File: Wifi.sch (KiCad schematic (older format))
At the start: 15 parts

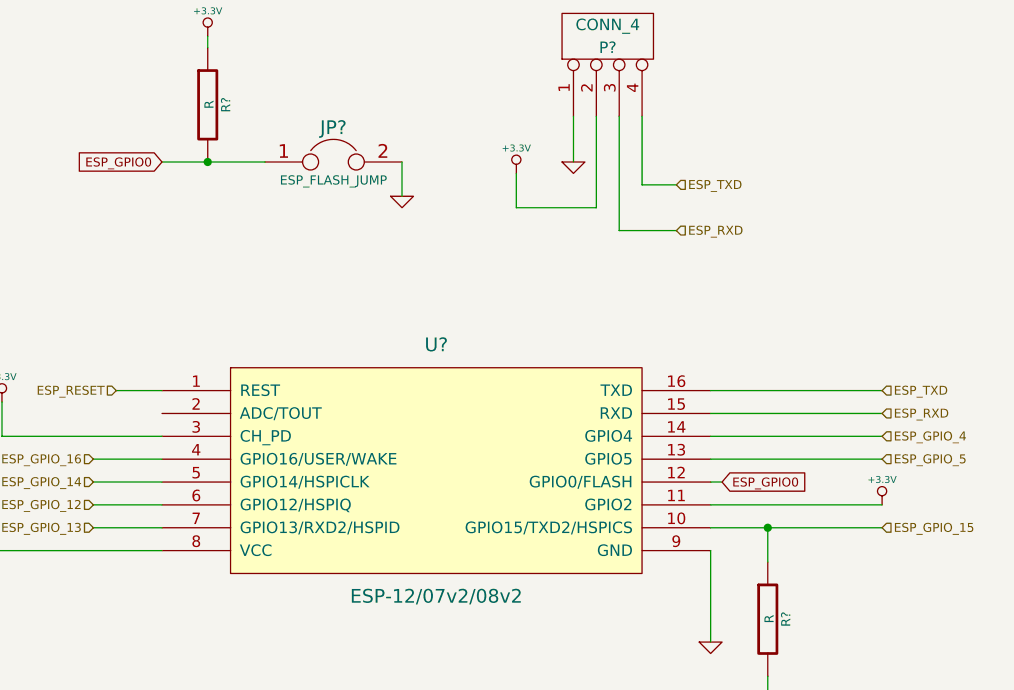
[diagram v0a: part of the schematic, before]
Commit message: Think sch finished
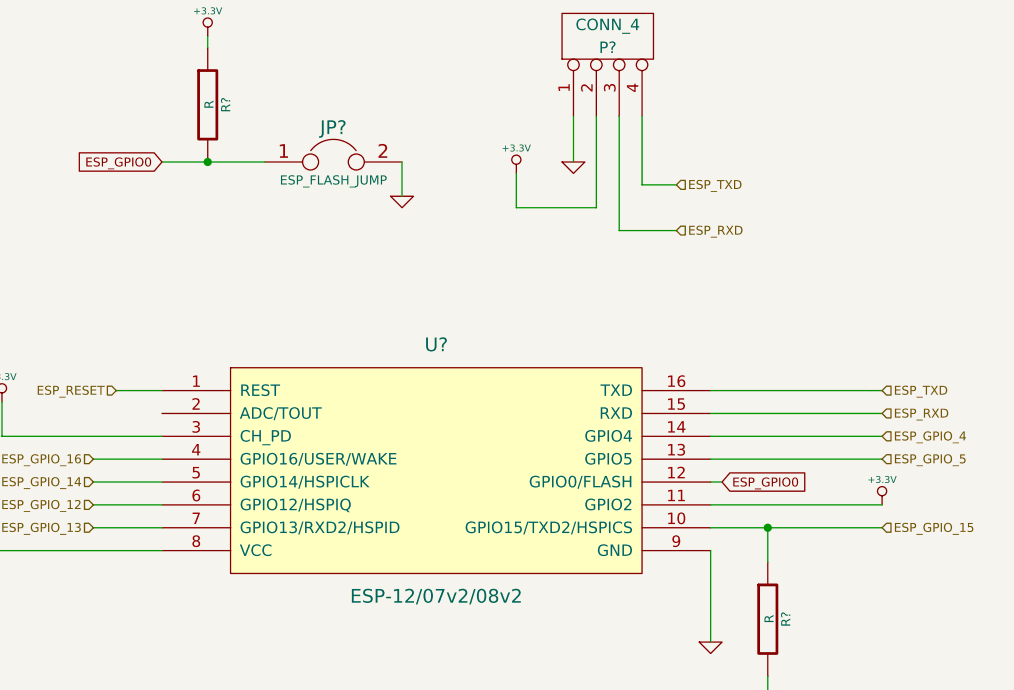
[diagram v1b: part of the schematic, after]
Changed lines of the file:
@@
 $EndComp
 $Comp
-L GND #PWR?
+L GND #PWR054
 U 1 1 55667722
 P 6650 2900
-F 0 "#PWR?" H 6650 2900 30  0001 C CNN
+F 0 "#PWR054" H 6650 2900 30  0001 C CNN
 F 1 "GND" H 6650 2830 30  0001 C CNN
 F 2 "" H 6650 2900 60  0000 C CNN
@@
 $EndComp
 $Comp
-L +3.3V #PWR?
+L +3.3V #PWR055
 U 1 1 55667729
 P 6400 2950
-F 0 "#PWR?" H 6400 2910 30  0001 C CNN
+F 0 "#PWR055" H 6400 2910 30  0001 C CNN
 F 1 "+3.3V" H 6400 3060 30  0000 C CNN
 F 2 "" H 6400 2950 60  0000 C CNN
@@
 $EndComp
 $Comp
-L +3.3V #PWR?
+L +3.3V #PWR056
 U 1 1 55667746
 P 5050 2350
-F 0 "#PWR?" H 5050 2310 30  0001 C CNN
+F 0 "#PWR056" H 5050 2310 30  0001 C CNN
 F 1 "+3.3V" H 5050 2460 30  0000 C CNN
 F 2 "" H 5050 2350 60  0000 C CNN
@@
 $EndComp
 $Comp
-L GND #PWR?
+L GND #PWR057
 U 1 1 5566774C
 P 5900 3050
-F 0 "#PWR?" H 5900 3050 30  0001 C CNN
+F 0 "#PWR057" H 5900 3050 30  0001 C CNN
 F 1 "GND" H 5900 2980 30  0001 C CNN
 F 2 "" H 5900 3050 60  0000 C CNN
@@
 ESP8266 Wifi Module
 $Comp
-L +3.3V #PWR?
+L +3.3V #PWR058
 U 1 1 5566775A
 P 8000 4400
-F 0 "#PWR?" H 8000 4360 30  0001 C CNN
+F 0 "#PWR058" H 8000 4360 30  0001 C CNN
 F 1 "+3.3V" H 8000 4510 30  0000 C CNN
 F 2 "" H 8000 4400 60  0000 C CNN
@@
 $EndComp
 $Comp
-L +3.3V #PWR?
+L +3.3V #PWR059
 U 1 1 55667760
 P 4150 3950
-F 0 "#PWR?" H 4150 3910 30  0001 C CNN
+F 0 "#PWR059" H 4150 3910 30  0001 C CNN
 F 1 "+3.3V" H 4150 4060 30  0000 C CNN
 F 2 "" H 4150 3950 60  0000 C CNN
@@
 $EndComp
 $Comp
-L GND #PWR?
+L GND #PWR060
 U 1 1 5566776E
 P 7500 5350
-F 0 "#PWR?" H 7500 5350 30  0001 C CNN
+F 0 "#PWR060" H 7500 5350 30  0001 C CNN
 F 1 "GND" H 7500 5280 30  0001 C CNN
 F 2 "" H 7500 5350 60  0000 C CNN
@@
 $EndComp
 $Comp
-L +3.3V #PWR?
+L +3.3V #PWR061
 U 1 1 5566915C
 P 2750 4500
-F 0 "#PWR?" H 2750 4460 30  0001 C CNN
+F 0 "#PWR061" H 2750 4460 30  0001 C CNN
 F 1 "+3.3V" H 2750 4610 30  0000 C CNN
 F 2 "" H 2750 4500 60  0000 C CNN
@@
 $EndComp
 $Comp
-L GND #PWR?
+L GND #PWR062
 U 1 1 556691BF
 P 7250 5000
-F 0 "#PWR?" H 7250 5000 30  0001 C CNN
+F 0 "#PWR062" H 7250 5000 30  0001 C CNN
 F 1 "GND" H 7250 4930 30  0001 C CNN
 F 2 "" H 7250 5000 60  0000 C CNN
@@
 $EndComp
 $Comp
-L GND #PWR?
+L GND #PWR063
 U 1 1 5566925F
 P 3200 5000
-F 0 "#PWR?" H 3200 5000 30  0001 C CNN
+F 0 "#PWR063" H 3200 5000 30  0001 C CNN
 F 1 "GND" H 3200 4930 30  0001 C CNN
 F 2 "" H 3200 5000 60  0000 C CNN
@@
 	5050 2350 5050 2400
 Wire Wire Line
-	4850 2900 5300 2900
+	4850 2900 5050 2900
+Wire Wire Line
+	5050 2900 5300 2900
 Wire Wire Line
 	5900 2900 5900 3050
@@
 	7250 4300 7300 4300
 Wire Wire Line
-	7250 4500 8000 4500
+	7250 4500 7500 4500
+Wire Wire Line
+	7500 4500 8000 4500
 Wire Wire Line
 	7500 4500 7500 4650
@@
 Text HLabel 7100 3000 2    39   Input ~ 0
 ESP_TXD
-Wire Wire Line
-	8000 4000 7250 4000
-Wire Wire Line
-	7250 3900 8000 3900
 Text HLabel 1600 7200 2    39   Input ~ 0
 ESP_TXD
@@
 Text HLabel 1600 7000 2    39   Input ~ 0
 ESP_GPIO_13
+Wire Wire Line
+	7250 3900 7950 3900
+Wire Wire Line
+	7950 3900 8000 3900
+Wire Wire Line
+	7250 4000 7650 4000
+Wire Wire Line
+	7650 4000 8000 4000
 $EndSCHEMATC
